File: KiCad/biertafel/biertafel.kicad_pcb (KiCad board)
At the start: 2 copper layers, 78.7 x 106.7 mm, 39 parts, among them J1 Screw_Terminal_01x02, J10 Screw_Terminal_01x02, J11 Raspberry connectors, J12 Screw_Terminal_01x02, J13 Raspberry connectors, J14 VCC socket, J2 Screw_Terminal_01x02, J3 Screw_Terminal_01x02, J4 Screw_Terminal_01x02, J5 Screw_Terminal_01x02, J6 Screw_Terminal_01x02, J7 Screw_Terminal_01x02, J8 Screw_Terminal_01x02, J9 Screw_Terminal_01x02, Q1 PN2222A, Q2 PN2222A, Q3 PN2222A, Q4 PN2222A, Q5 PN2222A, Q6 PN2222A

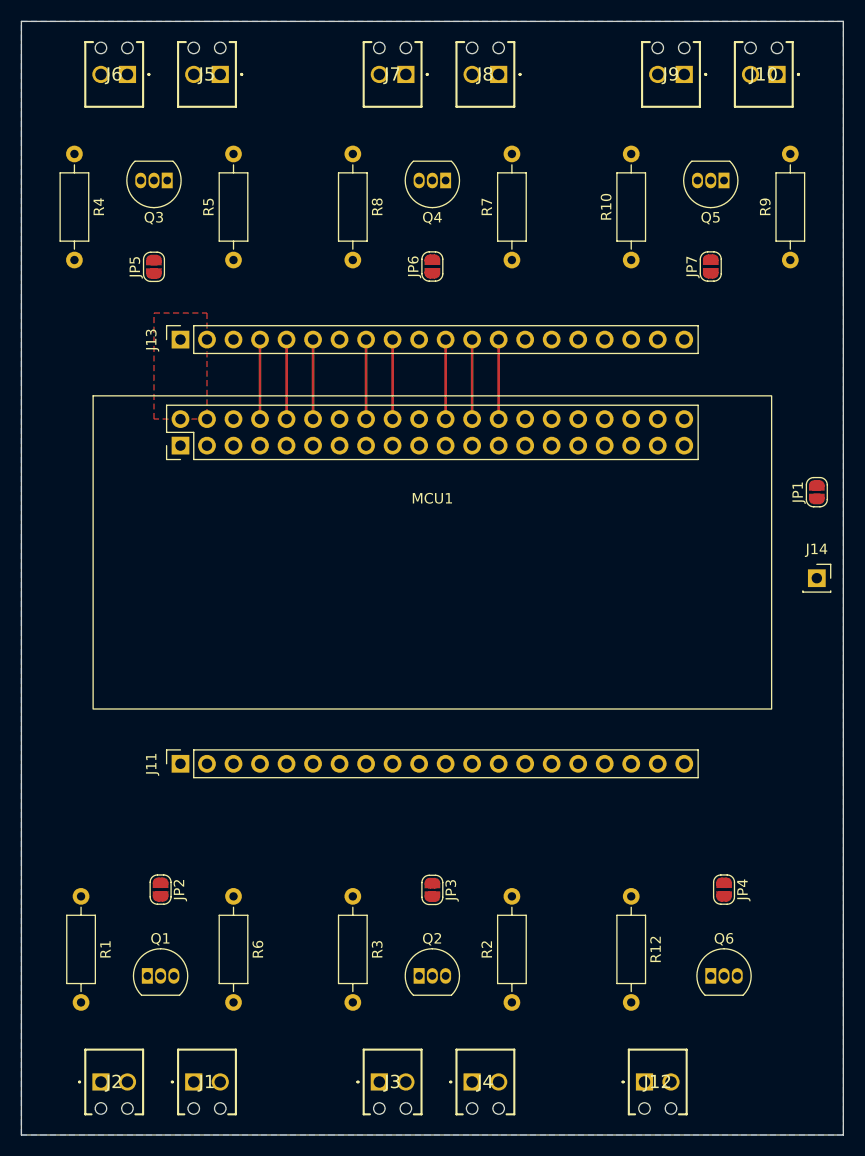
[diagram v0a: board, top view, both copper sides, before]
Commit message: PCB layout V0.1
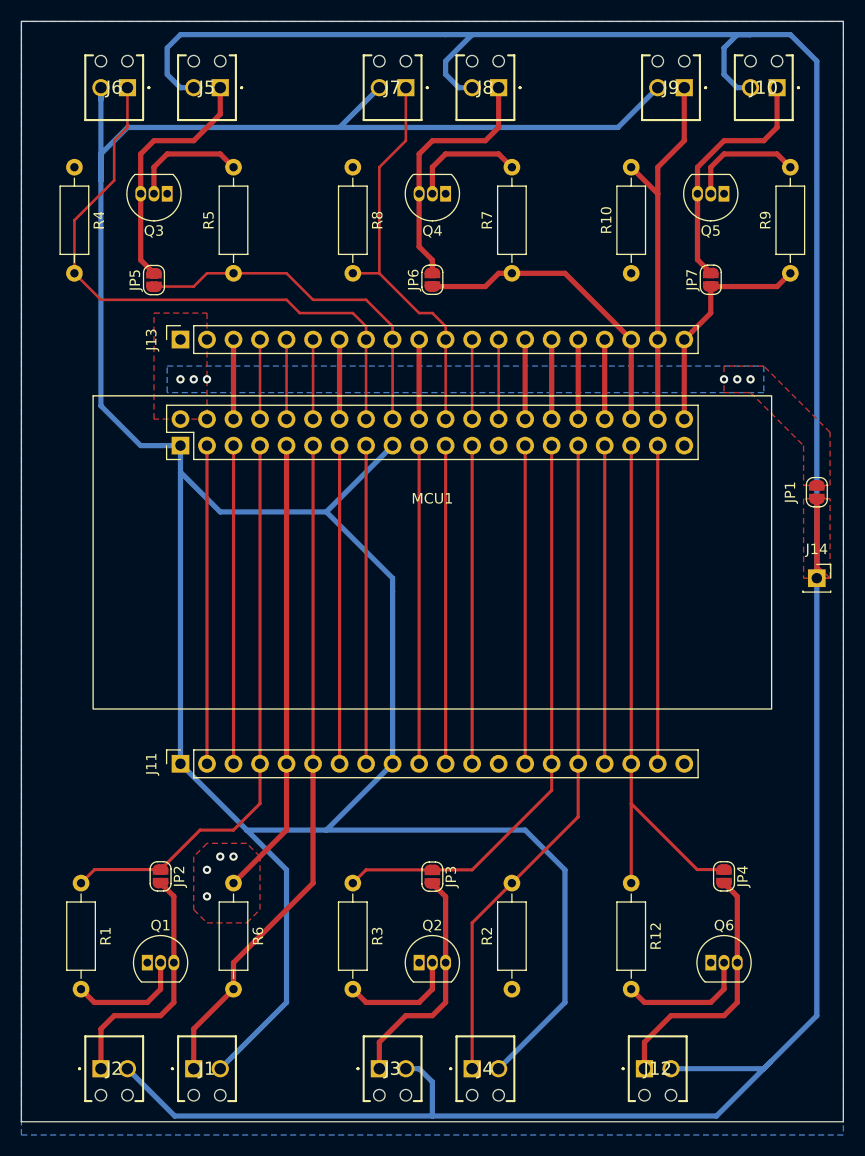
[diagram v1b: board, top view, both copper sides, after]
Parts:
- moved J1 1.27 mm to (120.7, 135.9)
- moved J12 1.27 mm to (163.8, 135.9)
- moved J2 1.27 mm to (111.8, 135.9)
- moved J3 1.27 mm to (138.4, 135.9)
- moved J4 1.27 mm to (147.3, 135.9)
- moved JP2 1.27 mm to (117.5, 117.5)
- moved JP3 1.27 mm to (143.5, 117.5)
- moved JP4 1.27 mm to (171.4, 117.5)
- moved JP5 1.27 mm to (116.8, 60.3)
- moved JP6 1.27 mm to (143.5, 60.3)
- moved JP7 1.27 mm to (170.2, 60.3)
- moved Q3 1.27 mm to (118.1, 52.1)
- moved Q4 1.27 mm to (144.8, 52.1)
- moved Q5 1.27 mm to (171.4, 52.1)
- moved R4 1.27 mm to (109.2, 49.5)
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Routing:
- net +3V3: track 0.00 -> 285.3 mm
- net VCC: track 0.00 -> 273.1 mm
- net GND: track 0.00 -> 82.1 mm, vias 0 -> 4
- net BUTTON1: track 0.00 -> 64.4 mm
- net BUTTON2: track 0.00 -> 63.9 mm
- net LED2: track 0.00 -> 55.8 mm
- net LED1: track 0.00 -> 54.6 mm
- net BUZZER: track 0.00 -> 53.4 mm
- net BUTTON3: track 7.62 -> 58.8 mm
- net BUTTON5: track 0.00 -> 36.4 mm
- net BUTTON4: track 7.62 -> 38.7 mm
- net SPI SCLK: track 0.00 -> 30.5 mm
- net SPI MOSI: track 0.00 -> 30.5 mm
- net SPI MISO: track 0.00 -> 30.5 mm
- net PWM GPIO13: track 0.00 -> 30.5 mm
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- added copper zone on B.Cu, net +5V
- added copper zone on F.Cu, net GND
- added copper zone on F.Cu, net VCC
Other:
- board size 78.7 x 106.7 mm -> 78.7 x 105.4 mm
